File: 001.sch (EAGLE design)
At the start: 26 parts, among them CN01 PWR5V, CN02 JD-VCC, CN03 TO-RLY, CN04 I2C-LCD, CN05 INPUT-A, CN06 INPUT-B, CN07 INPUT-C, CN08 BTN-A, CN09 BTN-B, CN10 BTN-C, CN11 BTN-STOP, CN12 DELAY-VR, M1 ARDUINO-NANO-3.0

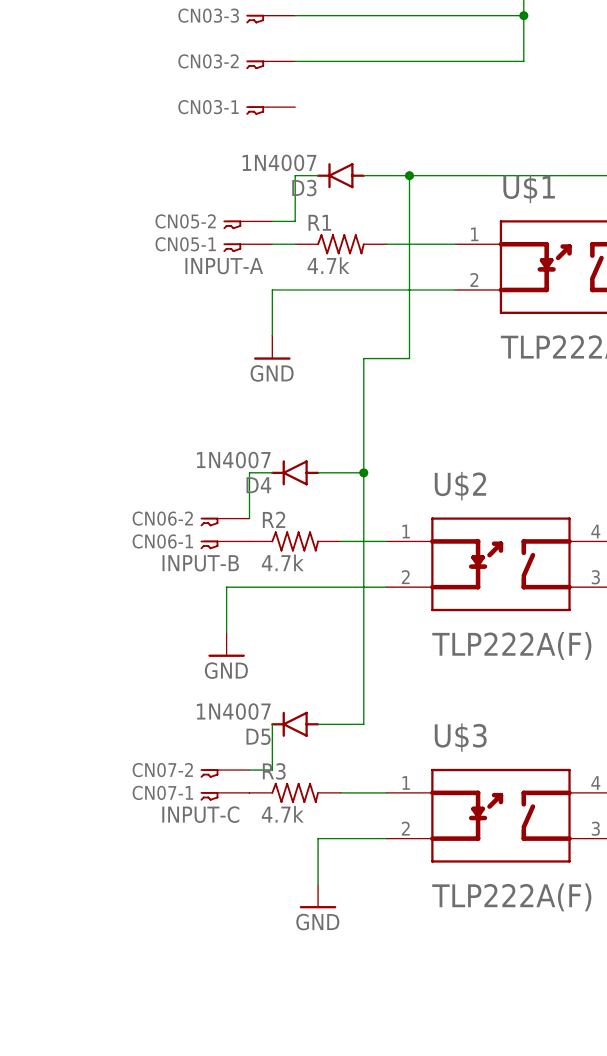
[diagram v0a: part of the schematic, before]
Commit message: ヴァリスタ追加
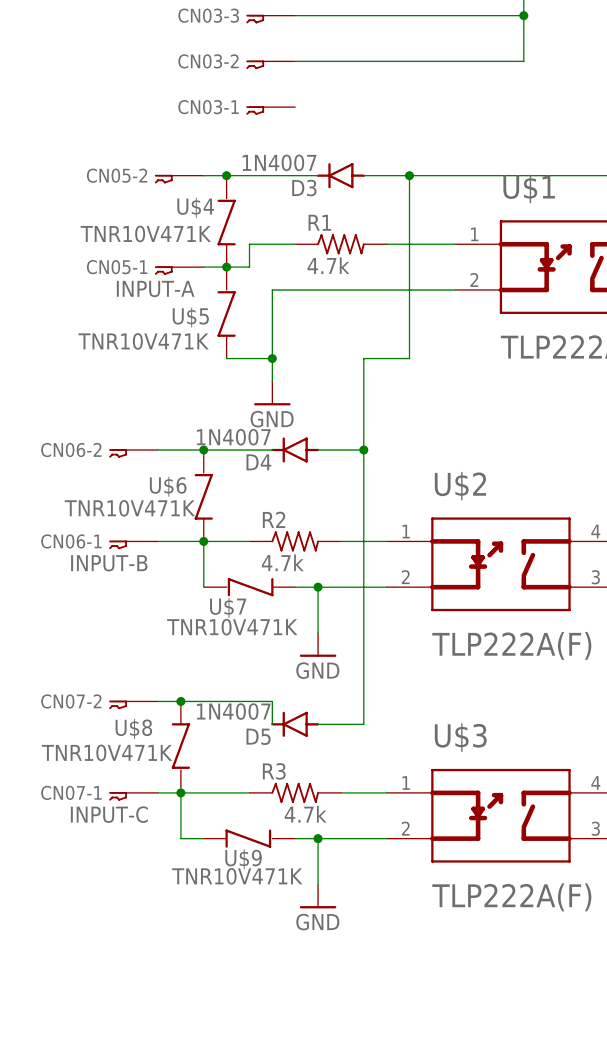
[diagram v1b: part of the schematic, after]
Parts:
- added U$4, U$5, U$6, U$7, U$8, U$9: TNR10V471K, holly:TNR10V471K
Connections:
- net GND: now also U$5.2, U$7.2, U$9.1
- net N$12: now also U$8.2
- net N$21: now also U$6.2, U$7.1
- net N$22: now also U$6.1
- net N$23: now also U$4.2, U$5.1
- net N$24: now also U$4.1
- net N$7: now also U$8.1, U$9.2
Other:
- moved on the sheet: CN05-1, CN05-2, CN06-1, CN06-2, CN07-1, CN07-2, D4
